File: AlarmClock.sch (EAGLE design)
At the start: 20 parts, among them IC1 LD1117AS33TR, T1 BC848

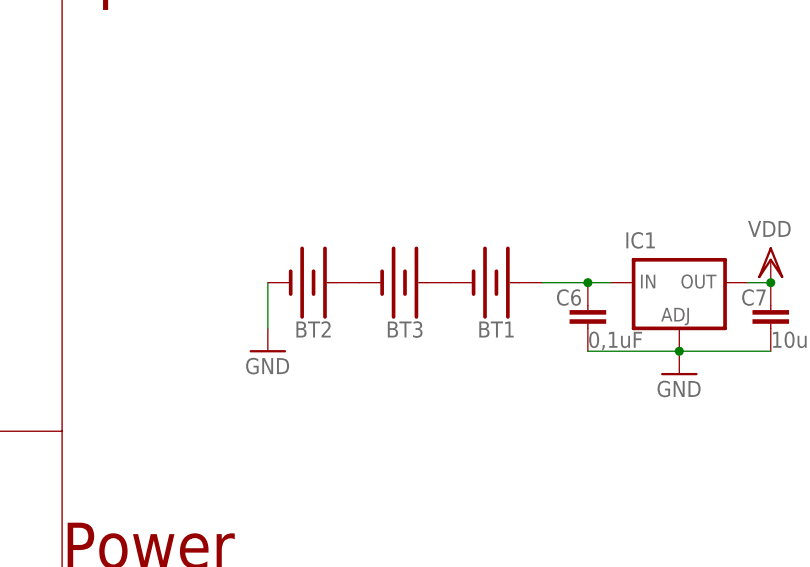
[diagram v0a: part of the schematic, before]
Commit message: Add files via upload
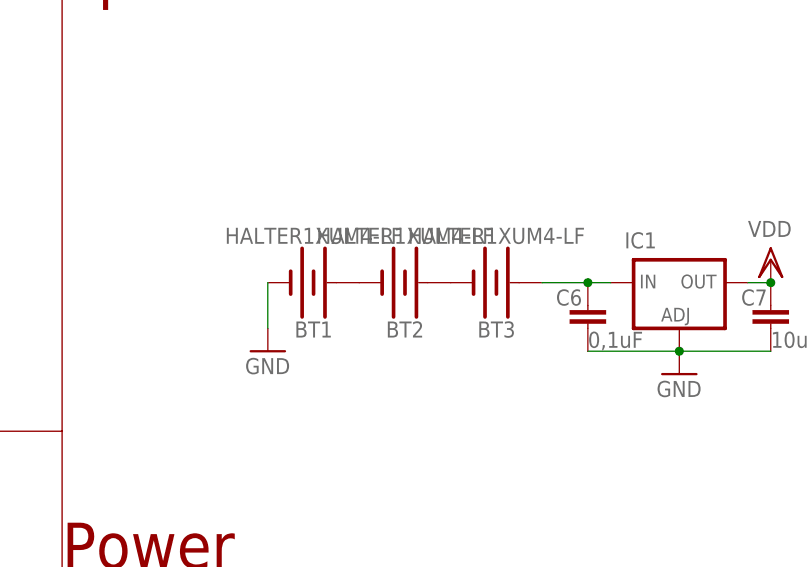
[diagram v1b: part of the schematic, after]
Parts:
- BT1, BT2, BT3: value (none) -> HALTER1XUM4-LF; device SparkFun-Batteries:BATTERY-AAA -> TheLibrary:HALTER1XUM4-LF
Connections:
- removed net N$6 (its old number): BT1.-, BT3.+
- new net N$5: BT1.+, BT2.-
- net GND: now also BT1.-; no longer BT2.-
- net VIN: now also BT3.+; no longer BT1.+
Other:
- moved on the sheet: BT1, BT2, BT3
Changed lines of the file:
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@@
 <part name="VDD3" library="supply1" library_urn="urn:adsk.eagle:library:371" deviceset="VDD" device=""/>
 <part name="VDD4" library="supply1" library_urn="urn:adsk.eagle:library:371" deviceset="VDD" device=""/>
-<part name="BT1" library="SparkFun-Batteries" deviceset="BATTERY" device="-AAA"/>
-<part name="BT2" library="SparkFun-Batteries" deviceset="BATTERY" device="-AAA"/>
+<part name="BT3" library="TheLibrary" deviceset="HALTER1XUM4-LF" device=""/>
+<part name="BT1" library="TheLibrary" deviceset="HALTER1XUM4-LF" device=""/>
 <part name="GND14" library="supply1" library_urn="urn:adsk.eagle:library:371" deviceset="GND" device=""/>
-<part name="BT3" library="SparkFun-Batteries" deviceset="BATTERY" device="-AAA"/>
+<part name="BT2" library="TheLibrary" deviceset="HALTER1XUM4-LF" device=""/>
 <part name="RST" library="rcl" library_urn="urn:adsk.eagle:library:334" deviceset="R-EU_" device="R1206" package3d_urn="urn:adsk.eagle:package:23540/2"/>
 <part name="SERIAL" library="pinhead-ext" deviceset="PINHD-1X5" device="_2.54-SMD-90°"/>
@@
 <attribute name="VALUE" x="238.76" y="72.39" size="1.778" layer="96"/>
 </instance>
-<instance part="BT1" gate="G$1" x="210.82" y="67.31" smashed="yes" rot="R180">
+<instance part="BT3" gate="G$1" x="210.82" y="67.31" smashed="yes" rot="R180">
 <attribute name="NAME" x="210.82" y="62.992" size="1.778" layer="95" font="vector" rot="R180" align="bottom-center"/>
 <attribute name="VALUE" x="210.82" y="71.628" size="1.778" layer="96" font="vector" rot="R180" align="top-center"/>
 </instance>
-<instance part="BT2" gate="G$1" x="190.5" y="67.31" smashed="yes" rot="R180">
+<instance part="BT1" gate="G$1" x="190.5" y="67.31" smashed="yes" rot="R180">
 <attribute name="NAME" x="190.5" y="62.992" size="1.778" layer="95" font="vector" rot="R180" align="bottom-center"/>
 <attribute name="VALUE" x="190.5" y="71.628" size="1.778" layer="96" font="vector" rot="R180" align="top-center"/>
@@
 <attribute name="VALUE" x="182.88" y="57.15" size="1.778" layer="96"/>
 </instance>
-<instance part="BT3" gate="G$1" x="200.66" y="67.31" smashed="yes" rot="R180">
+<instance part="BT2" gate="G$1" x="200.66" y="67.31" smashed="yes" rot="R180">
 <attribute name="NAME" x="200.66" y="62.992" size="1.778" layer="95" font="vector" rot="R180" align="bottom-center"/>
 <attribute name="VALUE" x="200.66" y="71.628" size="1.778" layer="96" font="vector" rot="R180" align="top-center"/>
@@
 <segment>
 <pinref part="GND14" gate="1" pin="GND"/>
-<pinref part="BT2" gate="G$1" pin="-"/>
+<pinref part="BT1" gate="G$1" pin="-"/>
 <wire x1="185.42" y1="62.23" x2="185.42" y2="67.31" width="0.1524" layer="91"/>
 </segment>
@@
 <pinref part="C6" gate="G$1" pin="2"/>
 <wire x1="223.52" y1="67.31" x2="220.98" y2="67.31" width="0.1524" layer="91"/>
-<pinref part="BT1" gate="G$1" pin="+"/>
+<pinref part="BT3" gate="G$1" pin="+"/>
 <wire x1="215.9" y1="67.31" x2="220.98" y2="67.31" width="0.1524" layer="91"/>
 <junction x="220.98" y="67.31"/>
@@
 <net name="N$5" class="0">
 <segment>
+<pinref part="BT1" gate="G$1" pin="+"/>
+<pinref part="BT2" gate="G$1" pin="-"/>
+</segment>
+</net>
+<net name="N$6" class="0">
+<segment>
+<pinref part="BT3" gate="G$1" pin="-"/>
 <pinref part="BT2" gate="G$1" pin="+"/>
-<pinref part="BT3" gate="G$1" pin="-"/>
-</segment>
-</net>
-<net name="N$6" class="0">
-<segment>
-<pinref part="BT1" gate="G$1" pin="-"/>
-<pinref part="BT3" gate="G$1" pin="+"/>
-</segment>
-</net>
+</segment>
+</net>
